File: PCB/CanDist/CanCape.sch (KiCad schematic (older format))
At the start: 15 parts, among them J1 Conn_01x02, J10 Conn_01x02, J11 Conn_01x02, J2 Conn_02x02_Top_Bottom, J3 Conn_02x02_Top_Bottom, J4 Conn_02x02_Top_Bottom, J5 Conn_02x02_Top_Bottom, J6 Conn_02x02_Top_Bottom, J7 Conn_02x02_Top_Bottom, J8 Conn_02x02_Top_Bottom, J9 Conn_02x02_Top_Bottom

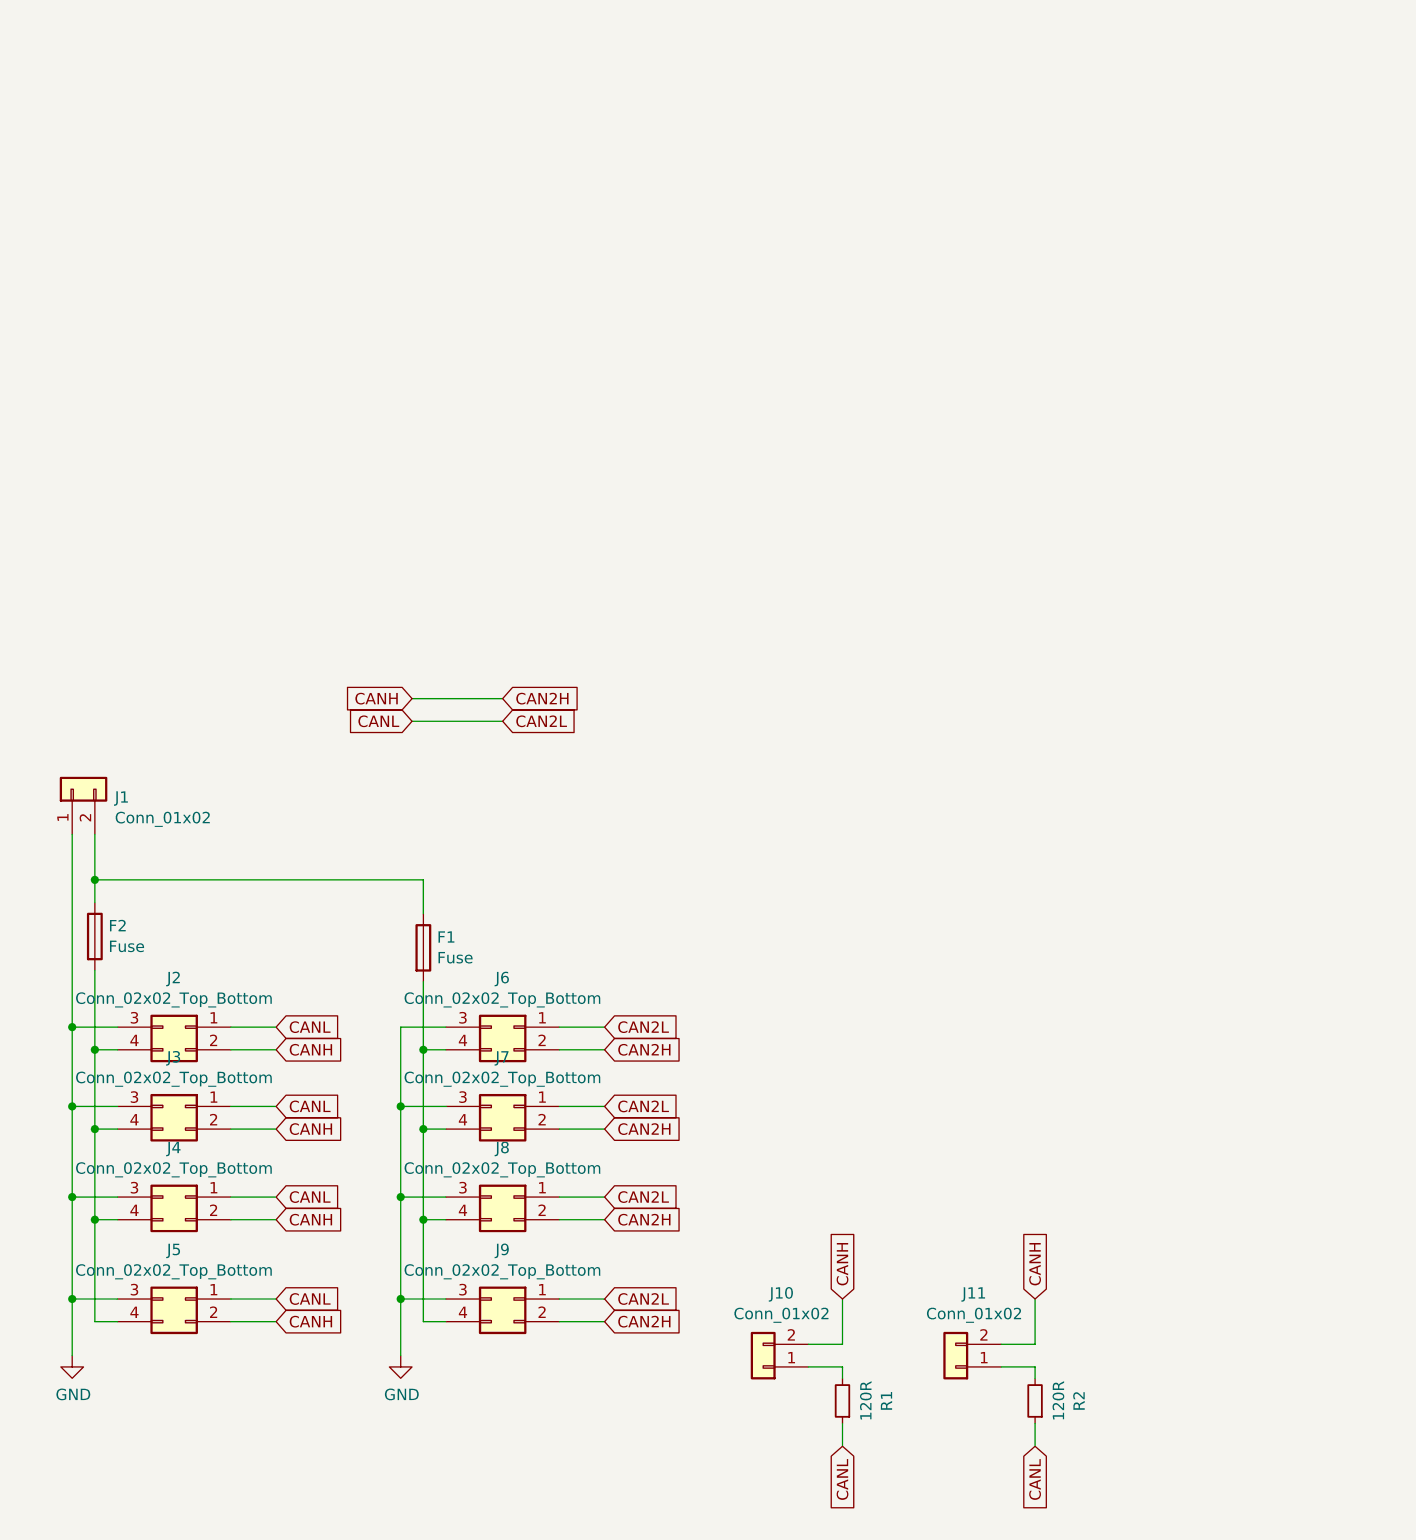
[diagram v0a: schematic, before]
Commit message: Added step file for Huvud v0.62
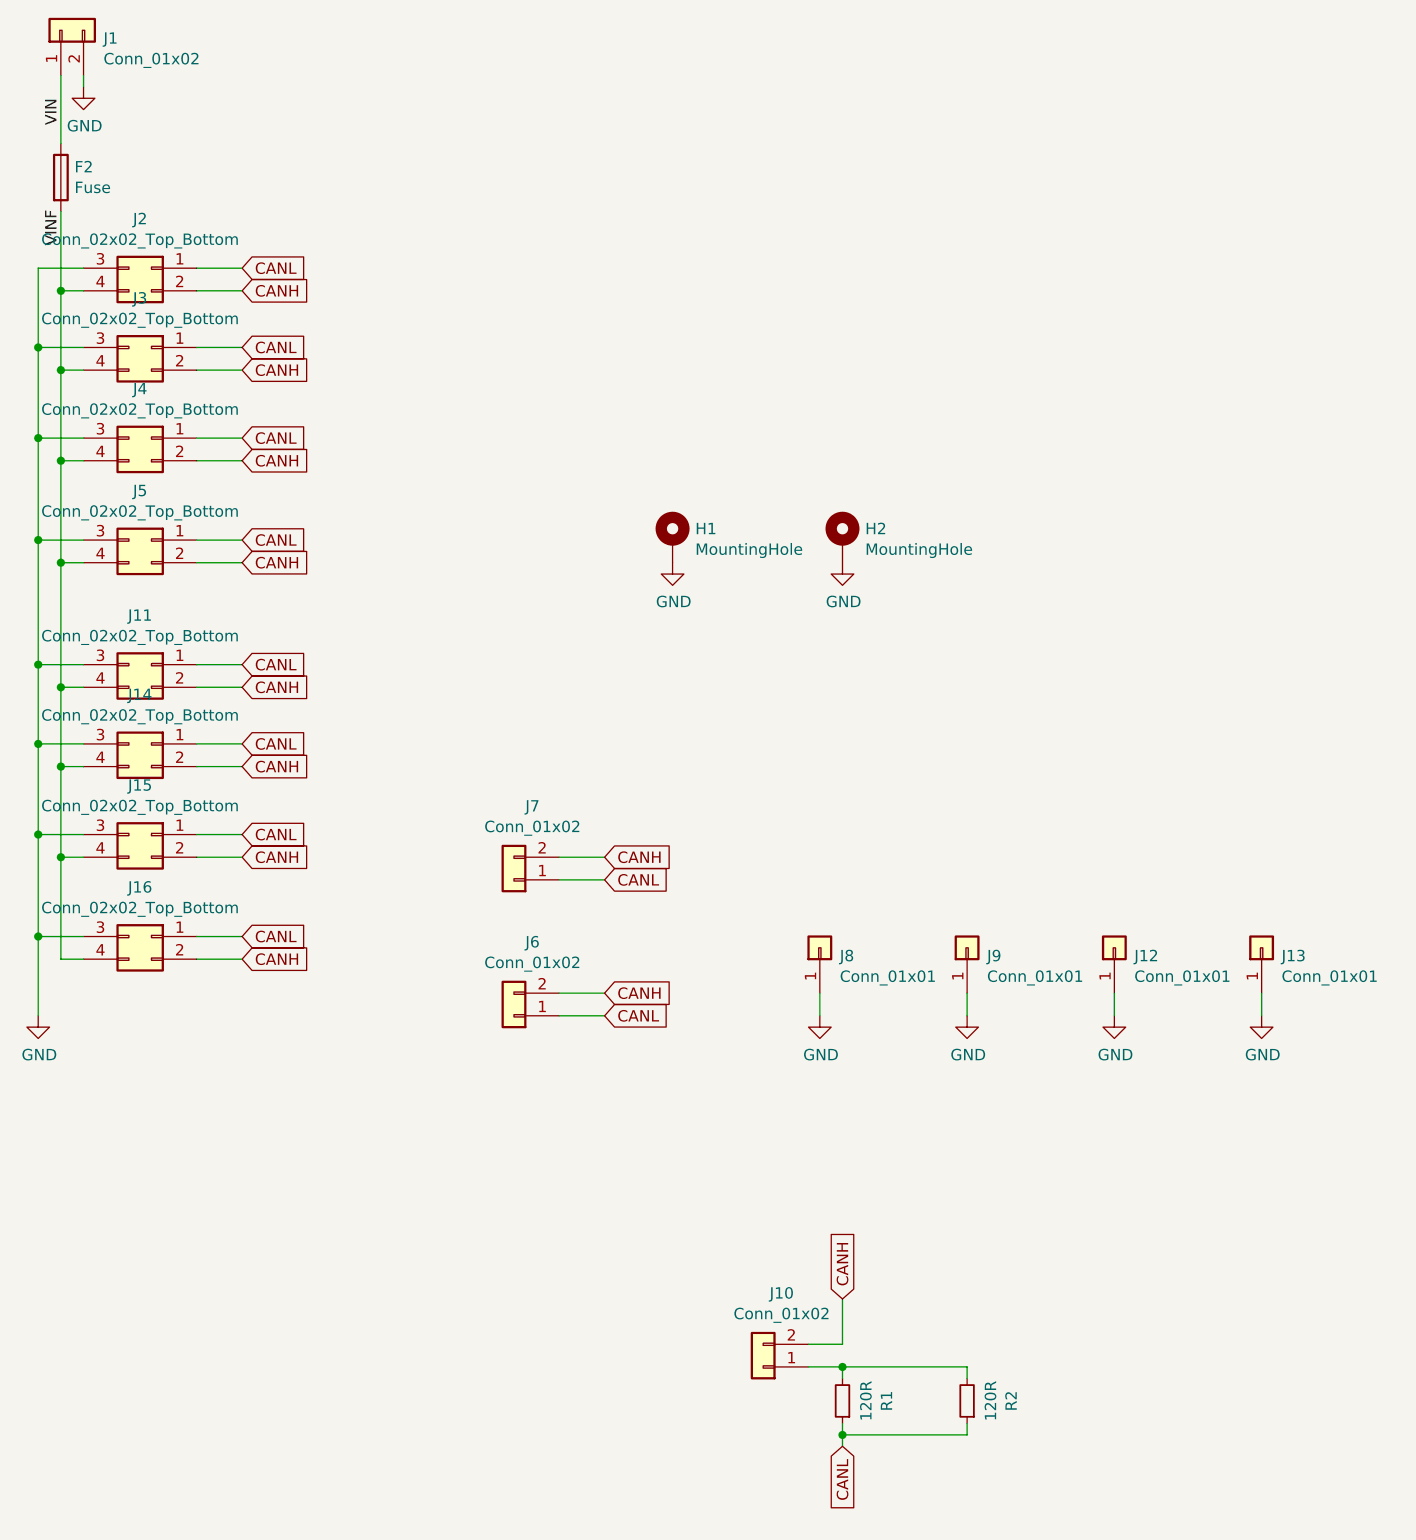
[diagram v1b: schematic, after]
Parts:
- removed F1: Fuse, cancape:3544-2_FuseHolder, symbol Device:Fuse
- removed J11: Conn_01x02, Connector_PinHeader_2.54mm:PinHeader_1x02_P2.54mm_Vertical, symbol Connector_Generic:Conn_01x02
- removed J6, J7, J8, J9: Conn_02x02_Top_Bottom, Connector_Molex:Molex_Micro-Fit_3.0_43045-0412_2x02_P3.00mm_Vertical, symbol Connector_Generic:Conn_02x02_Top_Bottom
- added H1, H2: MountingHole, MountingHole:MountingHole_3.2mm_M3_Pad_Via, symbol Mechanical:MountingHole_Pad
- added J11, J14, J15, J16: Conn_02x02_Top_Bottom, Connector_Molex:Molex_Micro-Fit_3.0_43045-0400_2x02_P3.00mm_Horizontal, symbol Connector_Generic:Conn_02x02_Top_Bottom
- added J12, J13, J8, J9: Conn_01x01, Connector_PinHeader_2.54mm:PinHeader_1x01_P2.54mm_Vertical, symbol Connector_Generic:Conn_01x01
- added J6, J7: Conn_01x02, Connector_JST:JST_XH_B2B-XH-A_1x02_P2.50mm_Vertical, symbol Connector_Generic:Conn_01x02
- F2: footprint cancape:3544-2_FuseHolder -> cancape:KEYSTONE-3568
- R2: footprint Resistor_SMD:R_0603_1608Metric -> Resistor_THT:R_Axial_DIN0207_L6.3mm_D2.5mm_P7.62mm_Horizontal; LCSC Part # C22787 -> (none)
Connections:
- net GND: now also J1.2 (Pin_2), H1.1, H2.1, J11.3 (Pin_3), J12.1 (Pin_1), J13.1 (Pin_1), J14.3 (Pin_3), J15.3 (Pin_3), J16.3 (Pin_3), J8.1 (Pin_1), J9.1 (Pin_1); no longer J1.1 (Pin_1)
- net VIN: now reaches F2.1
- net VIN: now also J1.1 (Pin_1); no longer J1.2 (Pin_2)
- net VINF: now reaches F2.2, J2.4 (Pin_4), J3.4 (Pin_4), J4.4 (Pin_4), J5.4 (Pin_4)
- net VINF: now also J11.4 (Pin_4), J14.4 (Pin_4), J15.4 (Pin_4), J16.4 (Pin_4)
- net at J10.1 (Pin_1), R1.2: now also R2.2
- net CAN2H renamed CANH
- net CANH: now also J11.2 (Pin_2), J14.2 (Pin_2), J15.2 (Pin_2), J16.2 (Pin_2), J6.2 (Pin_2), J7.2 (Pin_2)
- net CAN2L renamed CANL
- net CANL: now also J11.1 (Pin_1), J14.1 (Pin_1), J15.1 (Pin_1), J16.1 (Pin_1), J6.1 (Pin_1), J7.1 (Pin_1)
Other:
- moved on the sheet: F2, J1, J2, J3, J4, J5
